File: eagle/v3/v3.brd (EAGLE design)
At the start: 26.3 x 33 mm, 51 parts, among them IC1 MEGA8-AI

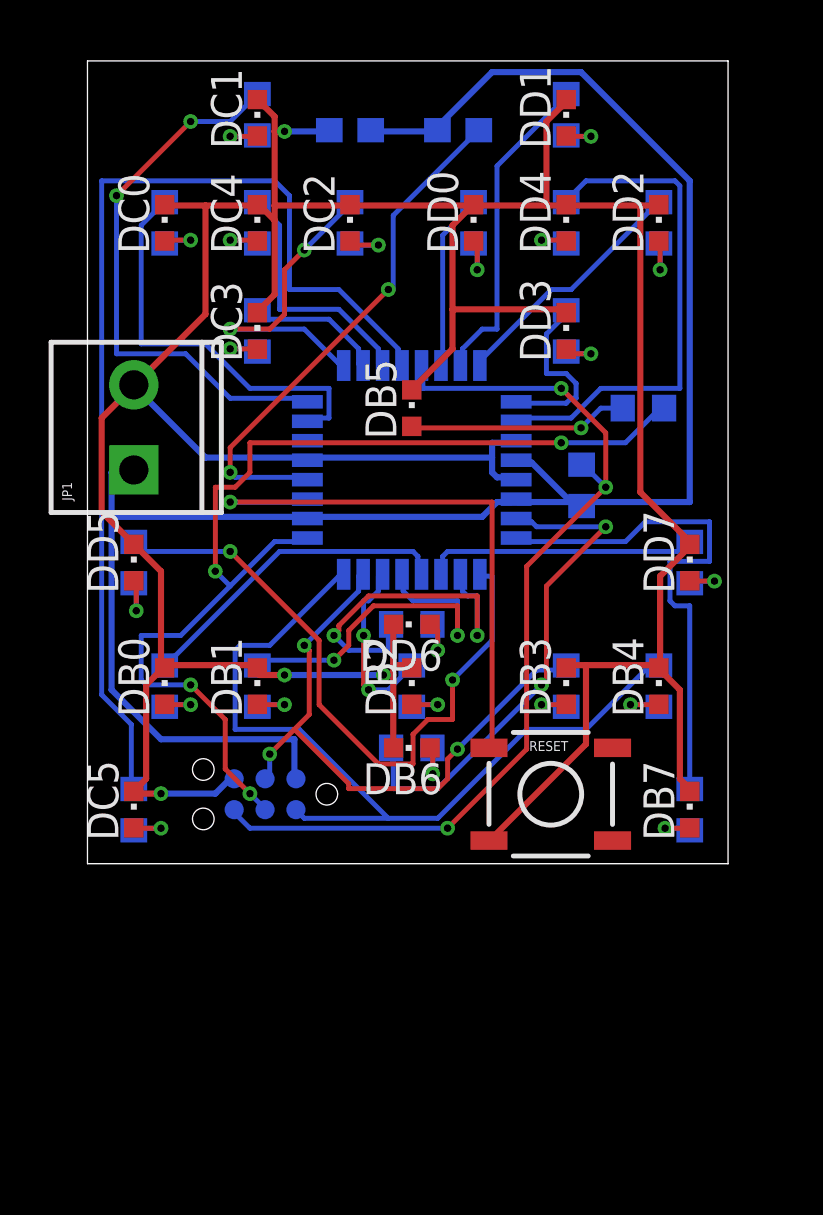
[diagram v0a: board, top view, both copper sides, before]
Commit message: Nouvelle version 0402 !!!!!!!!!!!!!
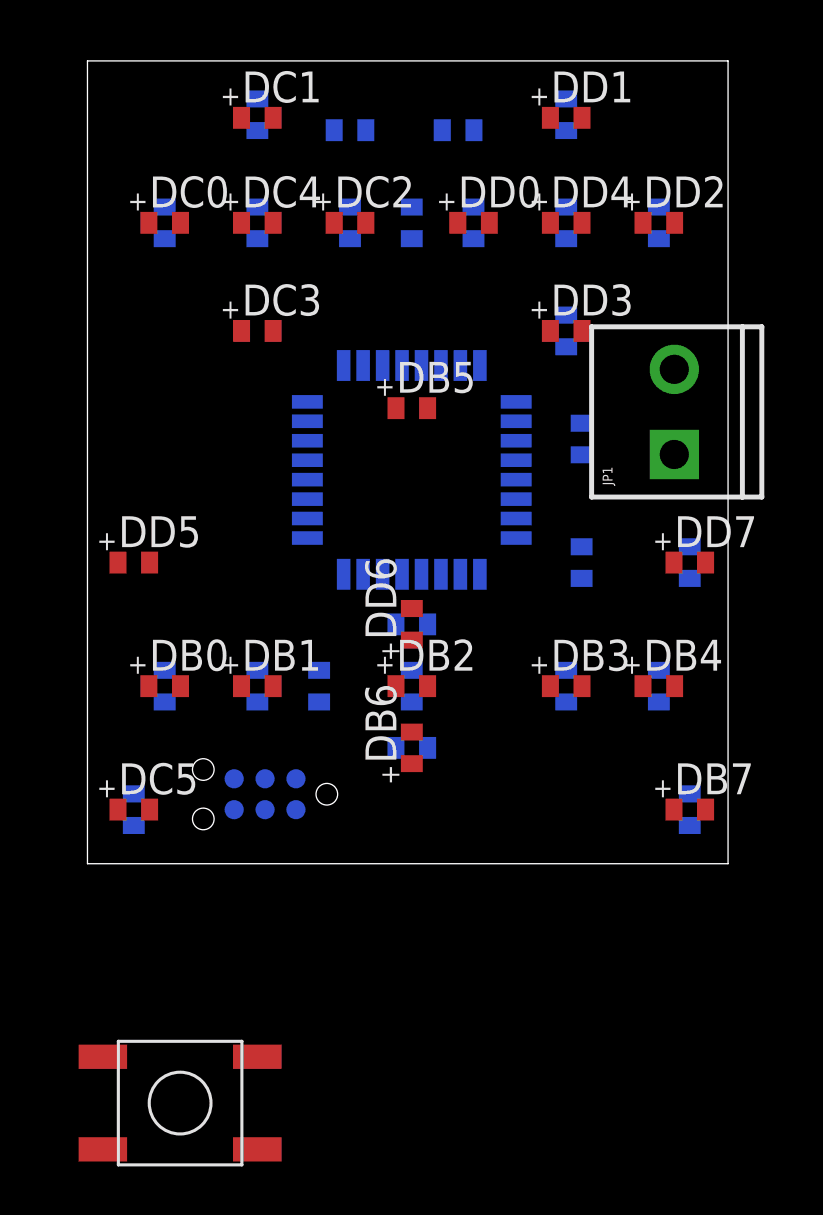
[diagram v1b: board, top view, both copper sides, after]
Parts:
- removed RESET: Reset uC, SparkFun:TACTILE_SWITCH_SMD
- added U$2: TEUCH4MM, florian:TEUCH4MM
- C1, C2: device eagle-ltspice:C0603 -> eagle-ltspice:C0402
- DB0, DB1, DB2, DB3, DB4, DB5, DB6, DB7, DC0, DC1, DC2, DC3, DC4, DC5, DD0, DD1, DD2, DD3, DD4, DD5, DD6, DD7: value (none) -> LED; device led:CHIPLED_0603 -> florian:D0402
- R1, RB0, RB1, RB2, RB3, RB4, RB5, RB6, RB7, RC0, RC1, RC2, RC3, RC4, RC5, RD0, RD1, RD2, RD3, RD4, RD5, RD6, RD7: device resistor:R0603 -> resistor:R0402
- moved JP1 22.2 mm to (24.8, 18.4)
- moved RD5 9.16 mm to (10.2, 8.89)
- moved RC3 7.75 mm to (14.0, 27.9)
- moved R1 3.17 mm to (21.0, 14.0)
- moved RB5 2.84 mm to (21.0, 19.1), turned to 90 degrees
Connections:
- new net N$22: U$2.1, U$2.4
- new net N$23: U$2.2, U$2.3
- net GND: no longer RESET.3
- net N$20: no longer RESET.1
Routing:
- net GND: track 156.3 -> 0.00 mm, vias 4 -> 0
- net +5V: track 77.1 -> 0.00 mm
- net N$8: track 43.7 -> 0.00 mm
- net SCK: track 43.7 -> 0.00 mm, vias 4 -> 0
- net RESET: track 38.7 -> 0.00 mm, vias 3 -> 0
- net MISO: track 34.5 -> 0.00 mm
- net N$13: track 27.0 -> 0.00 mm, vias 2 -> 0
- net MOSI: track 25.4 -> 0.00 mm, vias 3 -> 0
- net N$20: track 24.1 -> 0.00 mm, vias 1 -> 0
- net N$2: track 22.7 -> 0.00 mm, vias 2 -> 0
- net N$4: track 21.7 -> 0.00 mm, vias 2 -> 0
- net N$21: track 21.7 -> 0.00 mm
- net N$1: track 21.1 -> 0.00 mm, vias 2 -> 0
- net N$14: track 20.8 -> 0.00 mm
- net N$3: track 16.9 -> 0.00 mm
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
